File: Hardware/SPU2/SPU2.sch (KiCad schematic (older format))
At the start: 35 parts

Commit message: ich geh jz pennen gn :)
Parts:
- added D1, D2, D3, D4, D5, D6, D7, D8, D? (x8): LED, symbol Device:LED
- added R1, R2, R3, R4, R5, R6, R7, R8, R? (x8): R, symbol Device:R
- added U11, U12, U? (x2): 74LS173, symbol 74xx:74LS173
- added U13, U3, U?: 74LS245, symbol 74xx:74LS245
- gave numbers to parts that had none: 11
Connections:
- net labels added: CLK, D0, D1, D2, D3, D4, D5, D6, D7, DATA, ZERO, ~AI, ~AO, ~BI, ~BO, ~EO
- wire segments 166 -> 362
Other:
- note added: "ALU (LEDs)\n"
- note added: "ALU (output control)"
- note added: "REGISTER A\n"
- note added: "REGISTER B\n\n"
- moved on the sheet: U10A, U10B, U10C, U10D, U10E, U8A, U8B, U8C, U8D, U8E

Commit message: random push
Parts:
- removed U13, U?: 74LS245, symbol 74xx:74LS245
- added C? (x4): CP, symbol Device:CP
- added D? (x8): LED, symbol Device:LED
- added R? (x8): R, symbol Device:R
- added U? (x3): 74LS161, symbol 74xx:74LS161
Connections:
- net labels added: CE
- net labels removed: ~AO, ~BO
- wire segments 362 -> 406
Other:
- moved on the sheet: D1, D2, D3, D4, D5, D6, D7, D8, D?, R1, R2, R3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

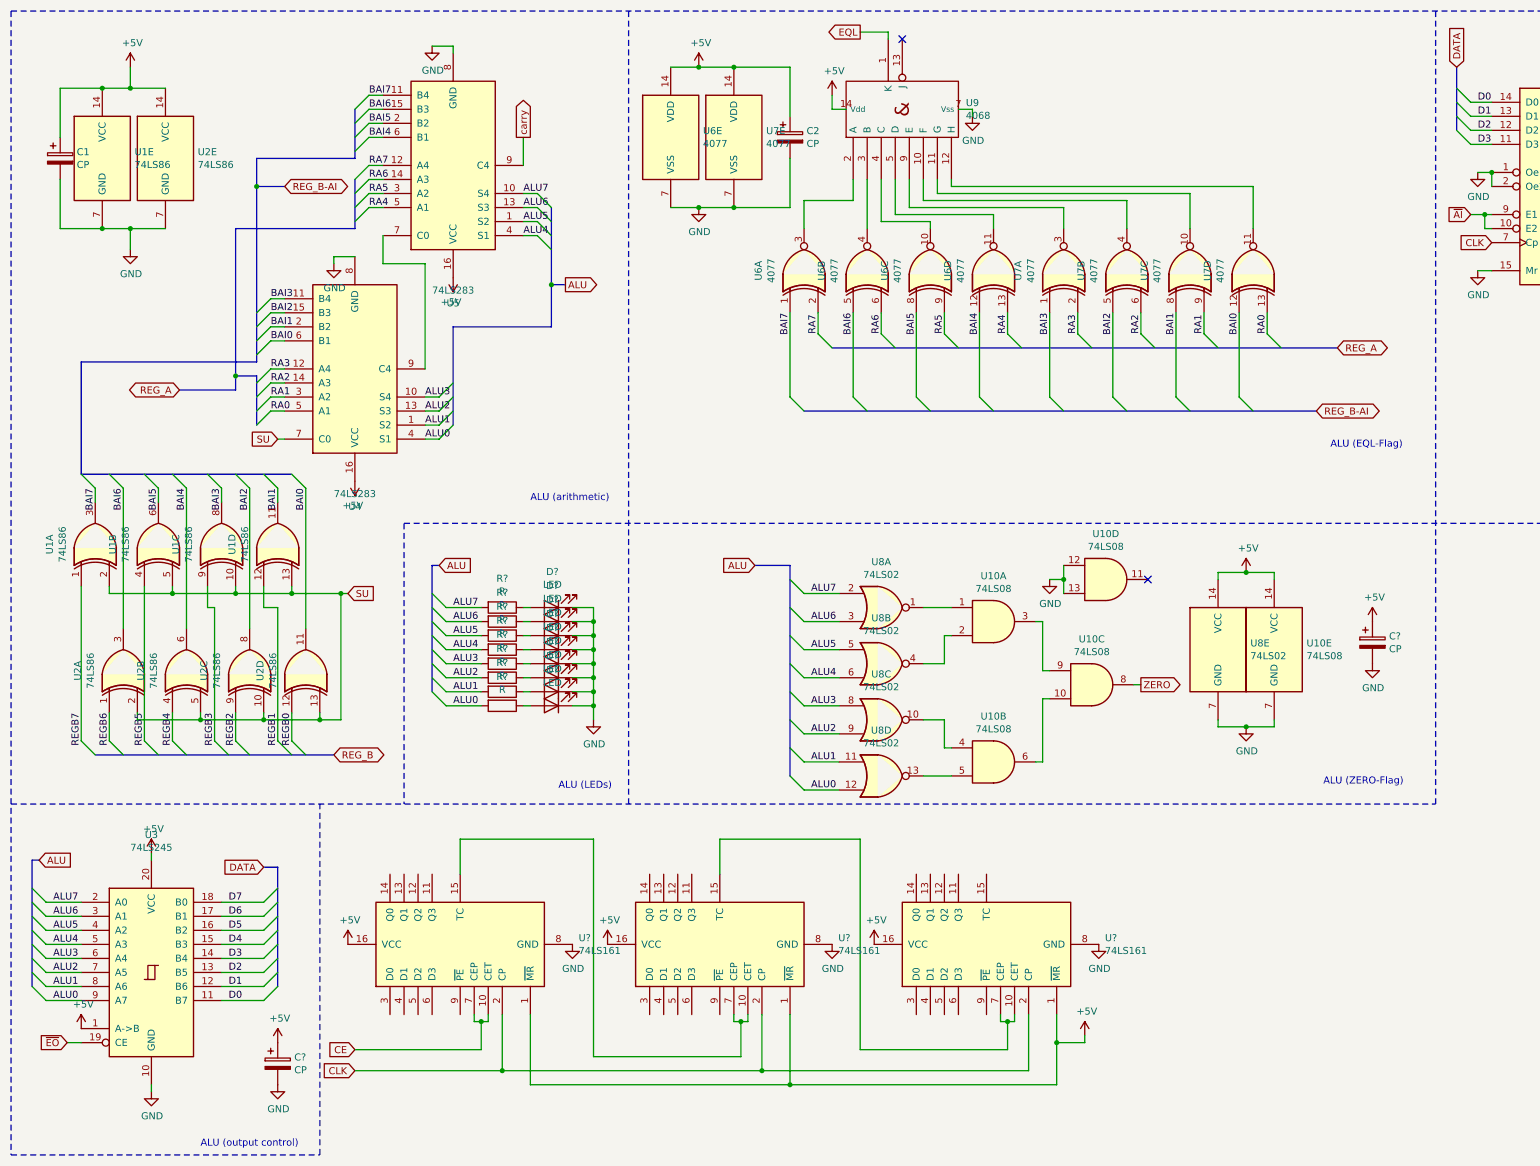
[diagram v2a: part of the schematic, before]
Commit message: foo
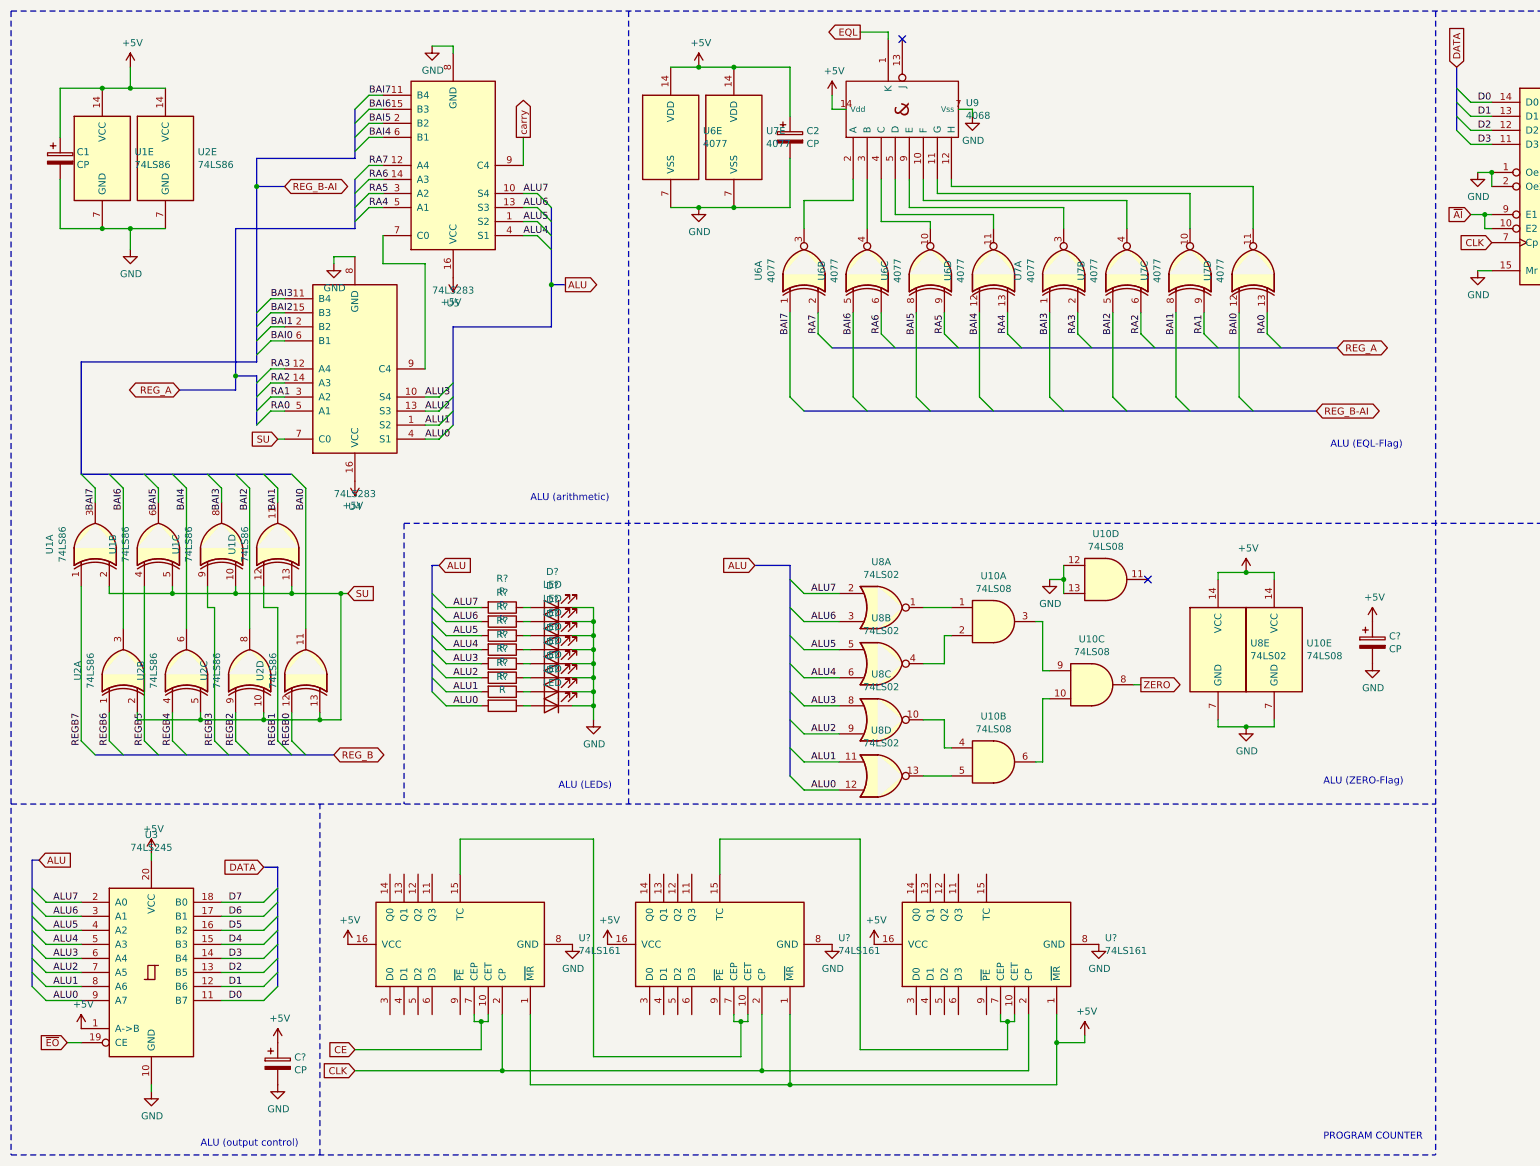
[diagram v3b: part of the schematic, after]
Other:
- note added: "PROGRAM COUNTER"
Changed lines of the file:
@@
 Wire Notes Line
 	1050 6450 11200 6450
-Wire Notes Line
-	11200 800  11200 6450
 Text Notes 10400 6400 0    50   ~ 0
 ALU (ZERO-Flag)\n\n
@@
 Wire Wire Line
 	2050 6800 2050 6850
-Wire Notes Line
-	1050 8950 3250 8950
 Wire Notes Line
 	3250 8950 3250 6450
@@
 Wire Wire Line
 	4400 8000 4350 8000
-Wire Bus Line
-	17650 1150 18350 1150
-Wire Bus Line
-	15600 1250 15600 1700
-Wire Bus Line
-	16800 2100 16800 2550
-Wire Bus Line
-	13400 1150 14100 1150
-Wire Bus Line
-	11350 1200 11350 1650
-Wire Bus Line
-	12550 2050 12550 2500
-Wire Bus Line
-	4050 4750 4050 5650
-Wire Bus Line
-	2950 6900 2950 7750
-Wire Bus Line
-	1200 6850 1200 7750
-Wire Bus Line
-	6600 4750 6600 6250
-Wire Bus Line
-	6900 3200 10500 3200
-Wire Bus Line
-	6700 3650 10350 3650
-Wire Bus Line
-	1650 6100 3350 6100
-Wire Bus Line
-	4200 3050 4200 3750
-Wire Bus Line
-	4900 2200 4900 2750
-Wire Bus Line
-	2800 3400 2800 3750
-Wire Bus Line
-	3500 2000 3500 2350
-Wire Bus Line
-	2800 2050 2800 3300
-Wire Bus Line
-	3500 1500 3500 1850
-Wire Bus Line
-	1550 4100 3050 4100
 $Comp
 L 74xx:74LS245 U3
@@
 	1    0    0    -1
 $EndComp
+Wire Notes Line
+	11200 800  11200 8950
+Wire Notes Line
+	1050 8950 11200 8950
+Wire Bus Line
+	15600 1250 15600 1700
+Wire Bus Line
+	16800 2100 16800 2550
+Wire Bus Line
+	11350 1200 11350 1650
+Wire Bus Line
+	12550 2050 12550 2500
+Wire Bus Line
+	4200 3050 4200 3750
+Wire Bus Line
+	4900 2200 4900 2750
+Wire Bus Line
+	2800 3400 2800 3750
+Wire Bus Line
+	3500 2000 3500 2350
+Wire Bus Line
+	3500 1500 3500 1850
+Wire Bus Line
+	1550 4100 3050 4100
+Wire Bus Line
+	2800 2050 2800 3300
+Wire Bus Line
+	13400 1150 14100 1150
+Wire Bus Line
+	17650 1150 18350 1150
+Wire Bus Line
+	4050 4750 4050 5650
+Wire Bus Line
+	2950 6900 2950 7750
+Wire Bus Line
+	1200 6850 1200 7750
+Wire Bus Line
+	6600 4750 6600 6250
+Wire Bus Line
+	6900 3200 10500 3200
+Wire Bus Line
+	6700 3650 10350 3650
+Wire Bus Line
+	1650 6100 3350 6100
+Text Notes 10400 8850 0    50   ~ 0
+PROGRAM COUNTER
 $EndSCHEMATC
